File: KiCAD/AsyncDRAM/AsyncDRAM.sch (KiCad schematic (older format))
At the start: 14 parts, among them J1 UART, J2 SPI, J3 UPDI, J4 POWER

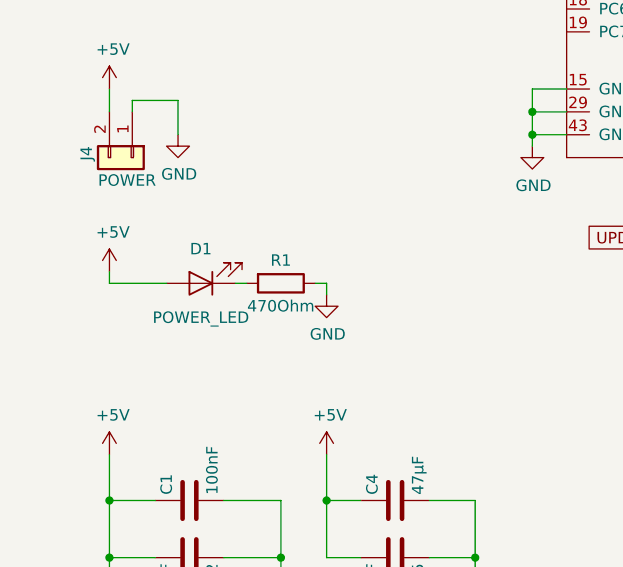
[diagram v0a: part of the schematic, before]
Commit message: Fixed LED finally
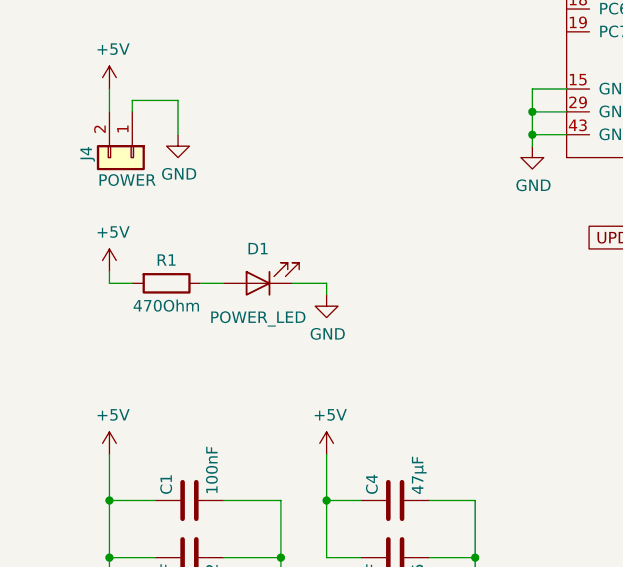
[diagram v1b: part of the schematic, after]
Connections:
- net +5V: now also R1.2; no longer D1.2 (A)
- net GND: now also D1.1 (K); no longer R1.1
- new net: D1.2 (A), R1.1
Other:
- moved on the sheet: D1, R1
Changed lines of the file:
@@
 L Device:LED D1
 U 1 1 5DADF535
-P 1050 5750
-F 0 "D1" H 1050 5600 50  0000 C CNN
-F 1 "POWER_LED" H 1050 5900 50  0000 C CNN
-F 2 "LEDSMD:LED_1206_3216Metric" H 1050 5750 50  0001 C CNN
-F 3 "~" H 1050 5750 50  0001 C CNN
-	1    1050 5750
+P 1300 5750
+F 0 "D1" H 1300 5600 50  0000 C CNN
+F 1 "POWER_LED" H 1300 5900 50  0000 C CNN
+F 2 "LEDSMD:LED_1206_3216Metric" H 1300 5750 50  0001 C CNN
+F 3 "~" H 1300 5750 50  0001 C CNN
+	1    1300 5750
 	-1   0    0    1
 $EndComp
@@
 L Device:R R1
 U 1 1 5DD94764
-P 1400 5750
-F 0 "R1" V 1300 5750 50  0000 C CNN
-F 1 "470Ohm" V 1500 5750 50  0000 C CNN
-F 2 "ResistorSMD:R_0805_2012Metric" V 1330 5750 50  0001 C CNN
-F 3 "~" H 1400 5750 50  0001 C CNN
-	1    1400 5750
+P 900 5750
+F 0 "R1" V 800 5750 50  0000 C CNN
+F 1 "470Ohm" V 1000 5750 50  0000 C CNN
+F 2 "ResistorSMD:R_0805_2012Metric" V 830 5750 50  0001 C CNN
+F 3 "~" H 900 5750 50  0001 C CNN
+	1    900  5750
 	0    1    1    0
 $EndComp
-Wire Wire Line
-	650  5750 650  5700
 Text Notes 3000 7250 0    50   ~ 0
 (PA5, PA6, PA7, PB0, PB1, PB2, PB3, PB4, PB5)
@@
 Wire Wire Line
 	4400 1300 3650 1300
-Wire Wire Line
-	1200 5750 1250 5750
-Wire Wire Line
-	1550 5750 1600 5750
-Wire Wire Line
-	1600 5750 1600 5800
-Wire Wire Line
-	650  5750 900  5750
 Text GLabel 3000 5550 0    50   Input ~ 0
 UPDI
@@
 Wire Wire Line
 	4100 4700 3950 4700
+Wire Wire Line
+	1050 5750 1150 5750
+Wire Wire Line
+	750  5750 650  5750
+Wire Wire Line
+	650  5750 650  5700
+Wire Wire Line
+	1450 5750 1600 5750
+Wire Wire Line
+	1600 5750 1600 5800
 $EndSCHEMATC

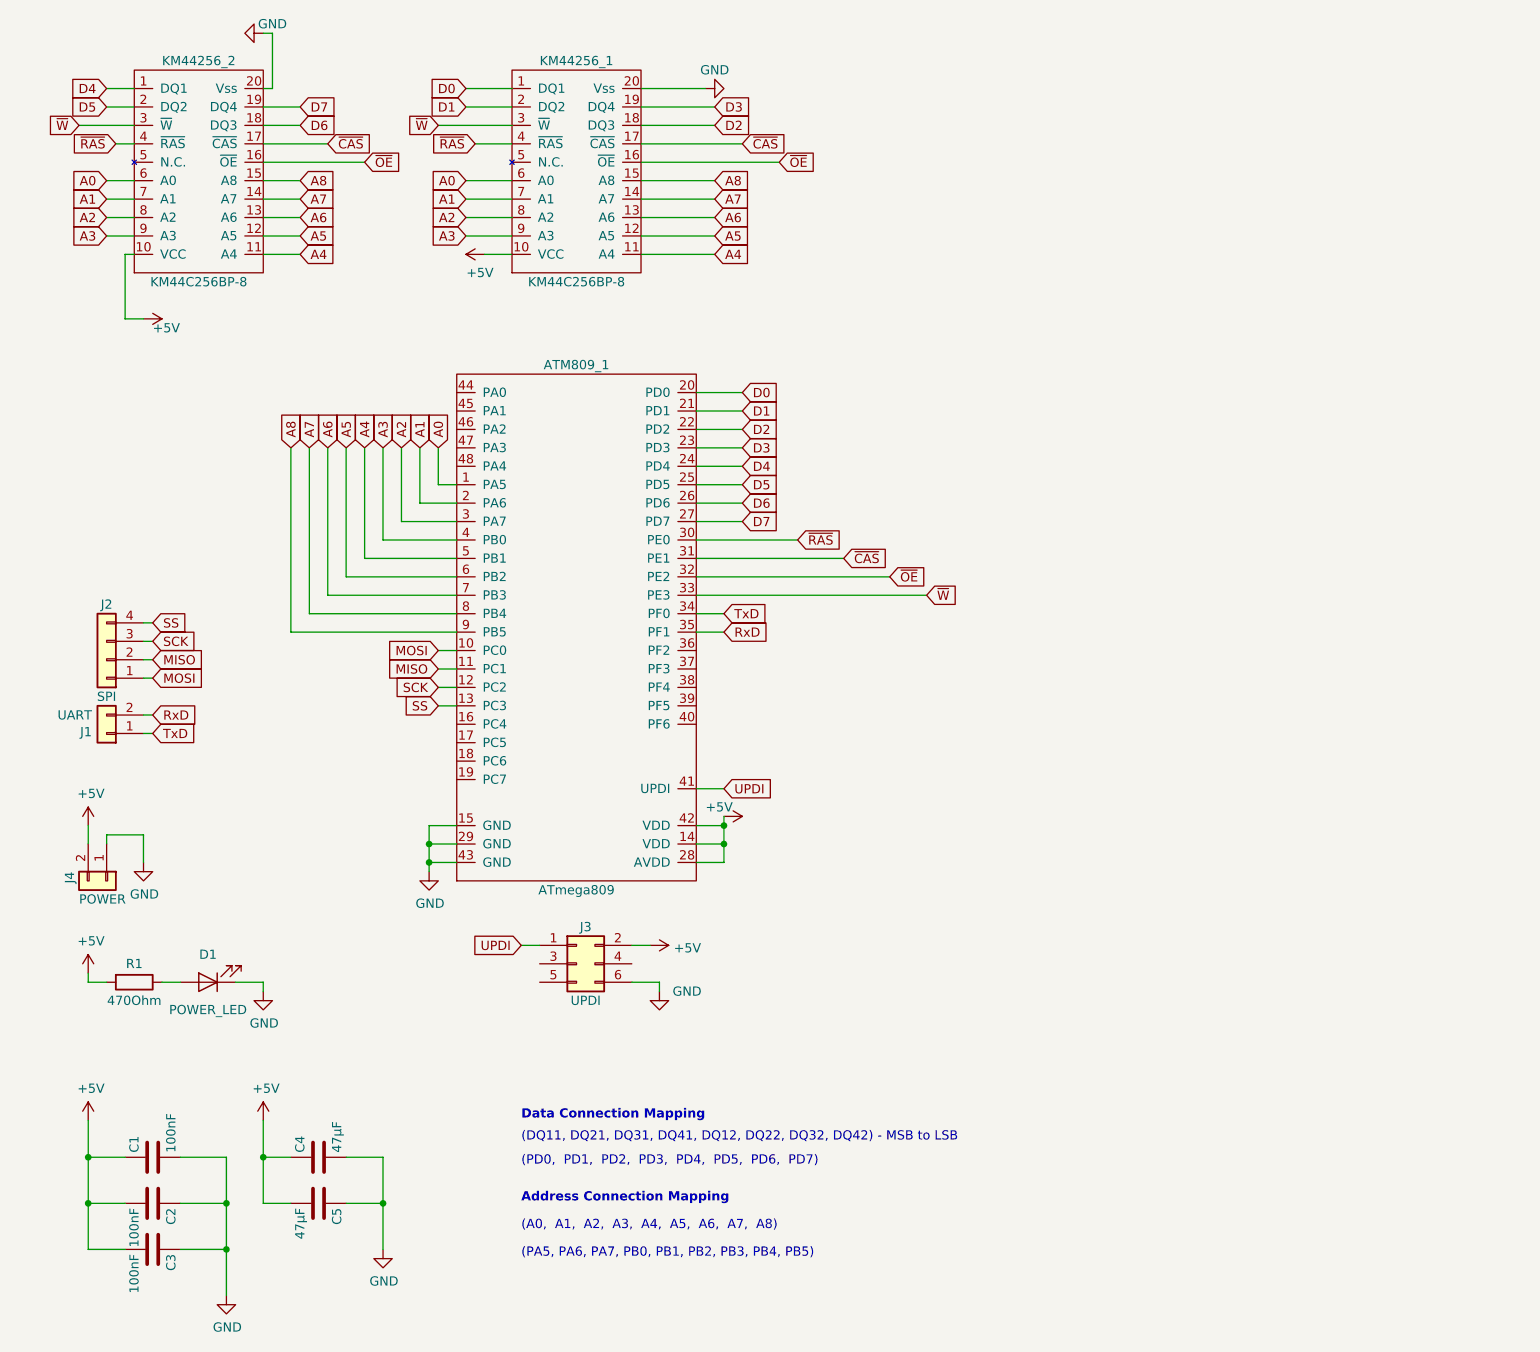
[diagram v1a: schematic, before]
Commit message: Update Praesi
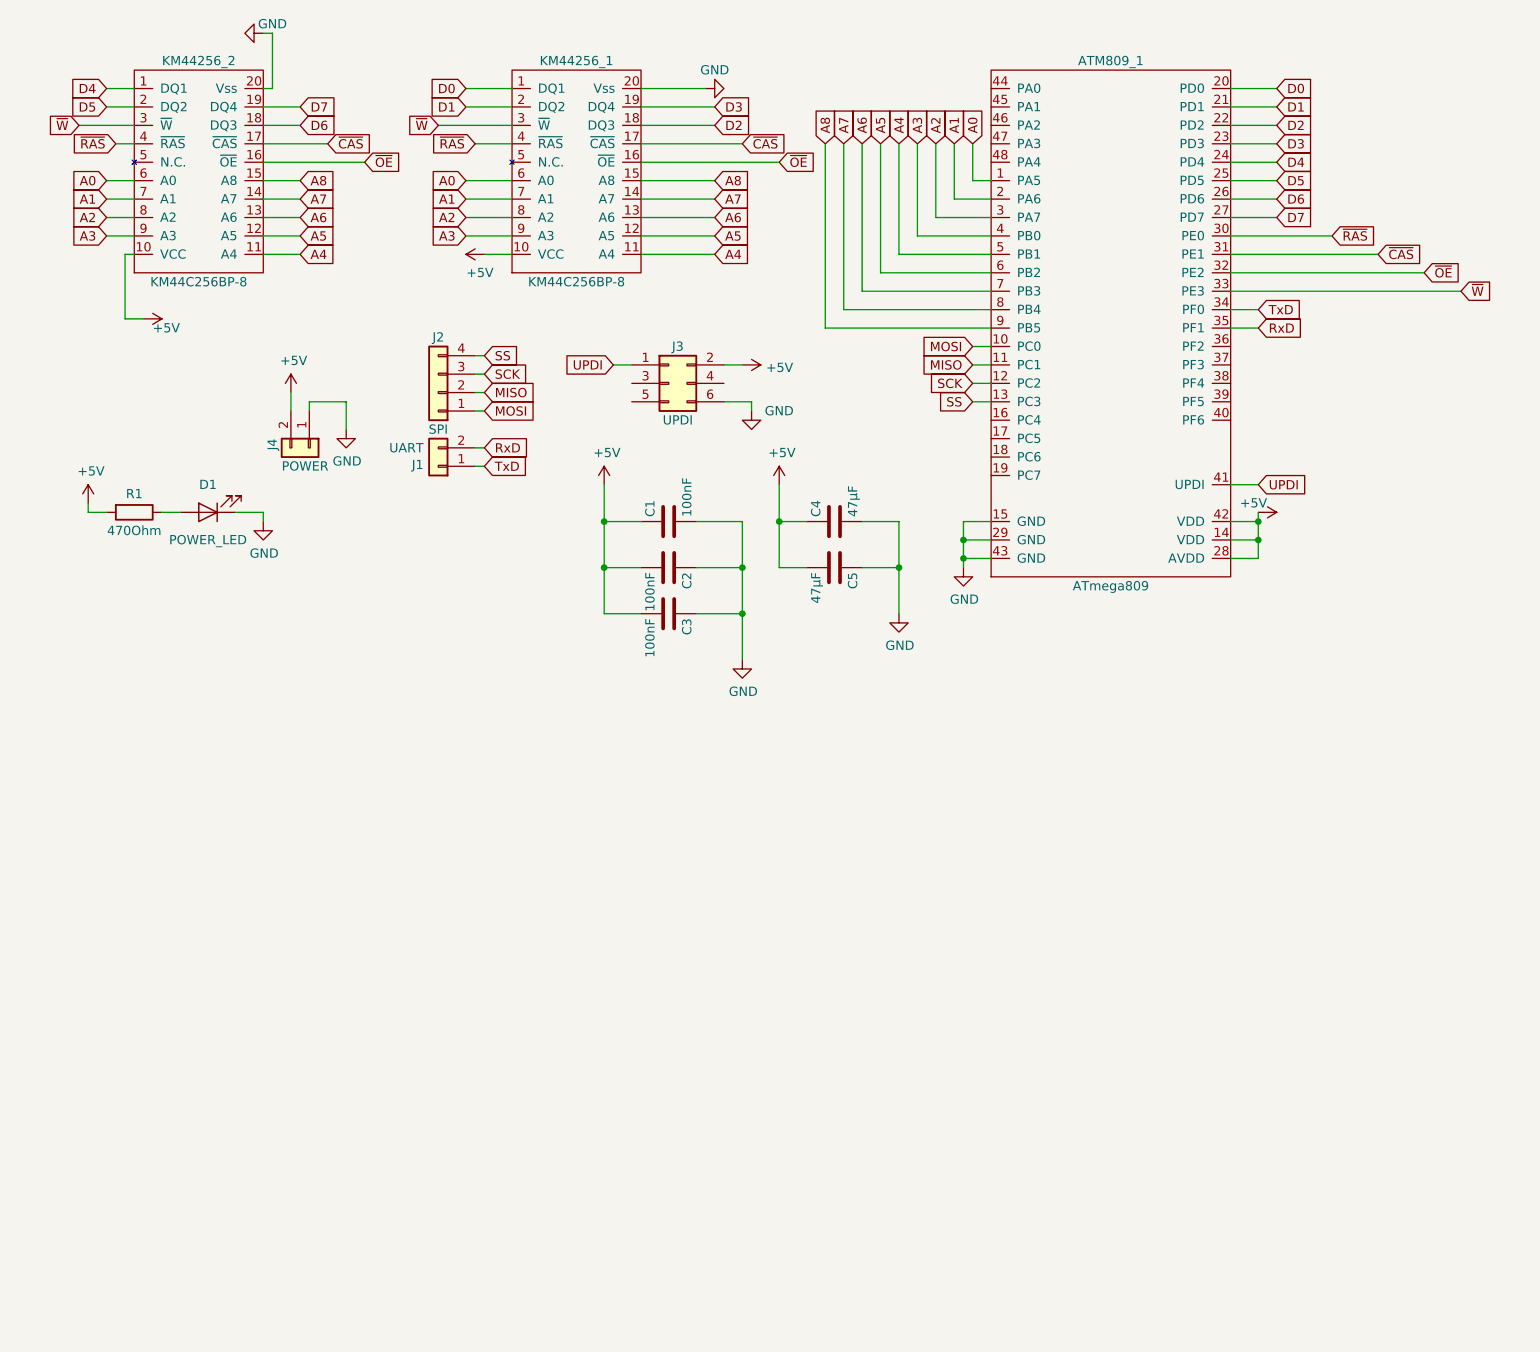
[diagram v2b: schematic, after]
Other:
- note removed: "(A0, A1, A2, A3, A4, A5, A6, A7, A8)"
- note removed: "(DQ11, DQ21, DQ31, DQ41, DQ12, DQ22, DQ32, DQ42) - MSB to LSB\n\n"
- note removed: "(PA5, PA6, PA7, PB0, PB1, PB2, PB3, PB4, PB5)"
- note removed: "(PD0, PD1, PD2, PD3, PD4, PD5, PD6, PD7)"
- note removed: "Address Connection Mapping"
- note removed: "Data Connection Mapping"
- moved on the sheet: ATM809_1, C1, C2, C3, C4, C5, D1, J1, J2, J3, J4, R1
